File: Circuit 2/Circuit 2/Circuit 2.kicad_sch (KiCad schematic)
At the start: 18 parts, among them SW1 SW_DIP_x08, SW2 SW_DIP_x08, U1 7408, U2 7485, U3 7432

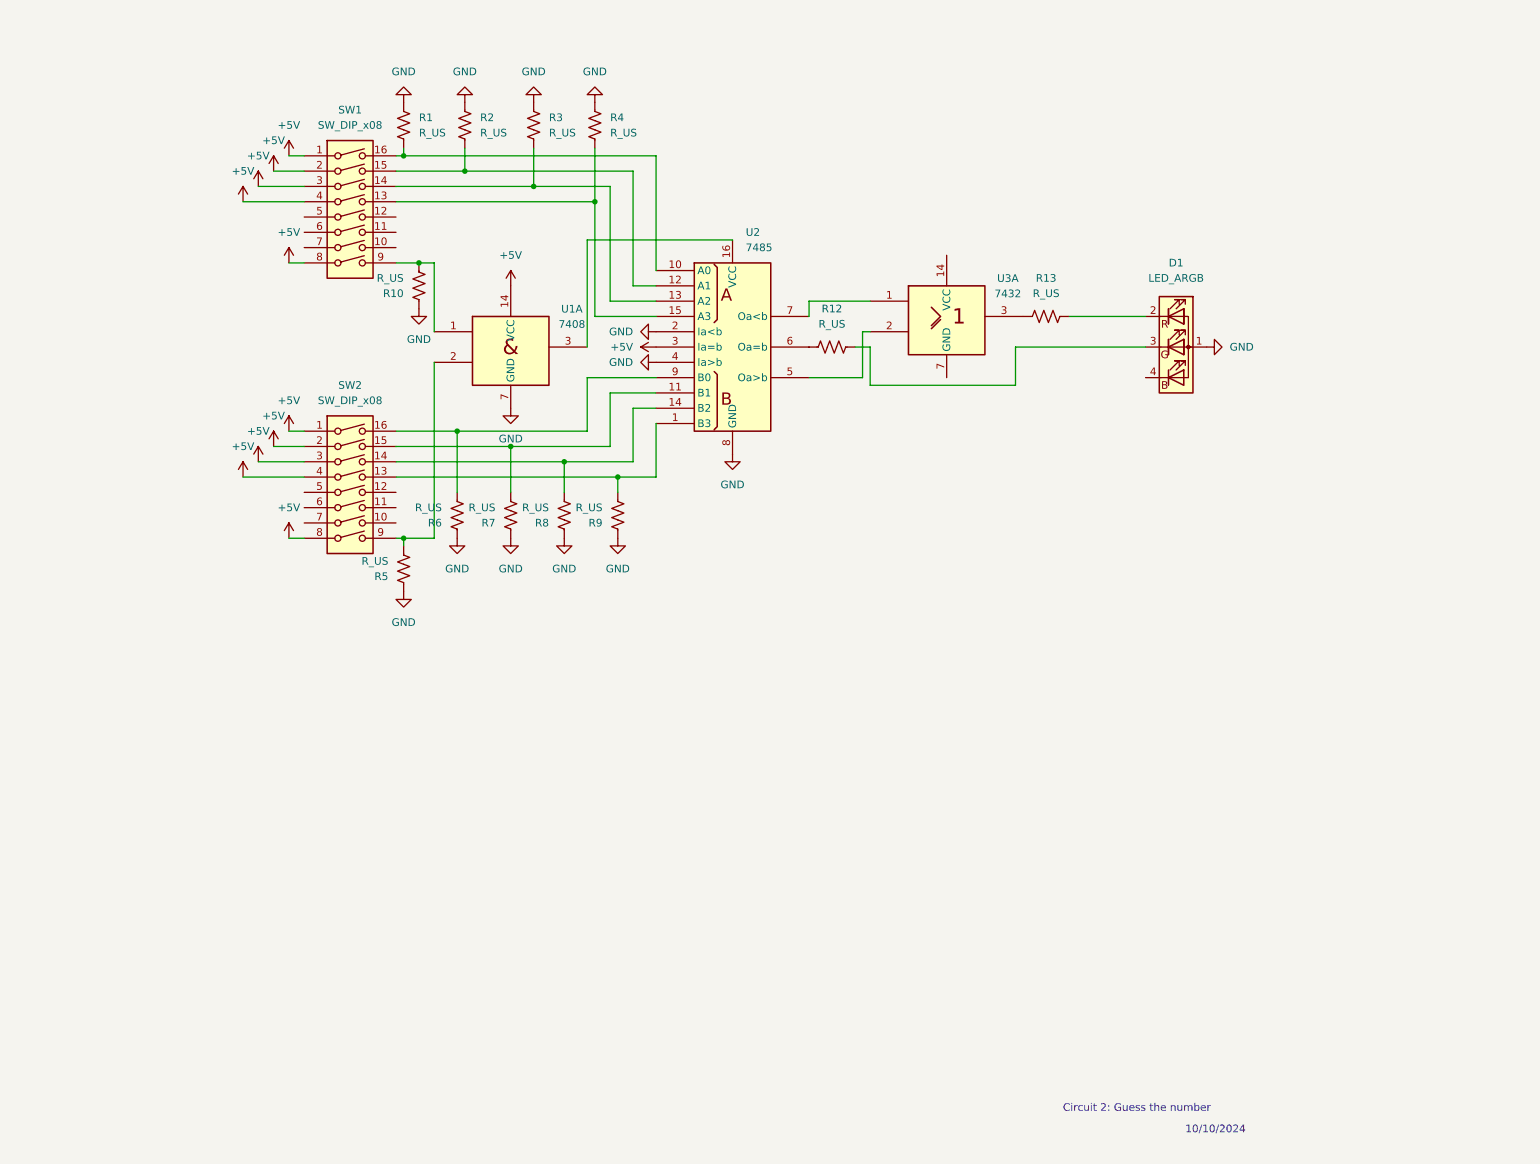
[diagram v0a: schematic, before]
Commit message: Add files via upload
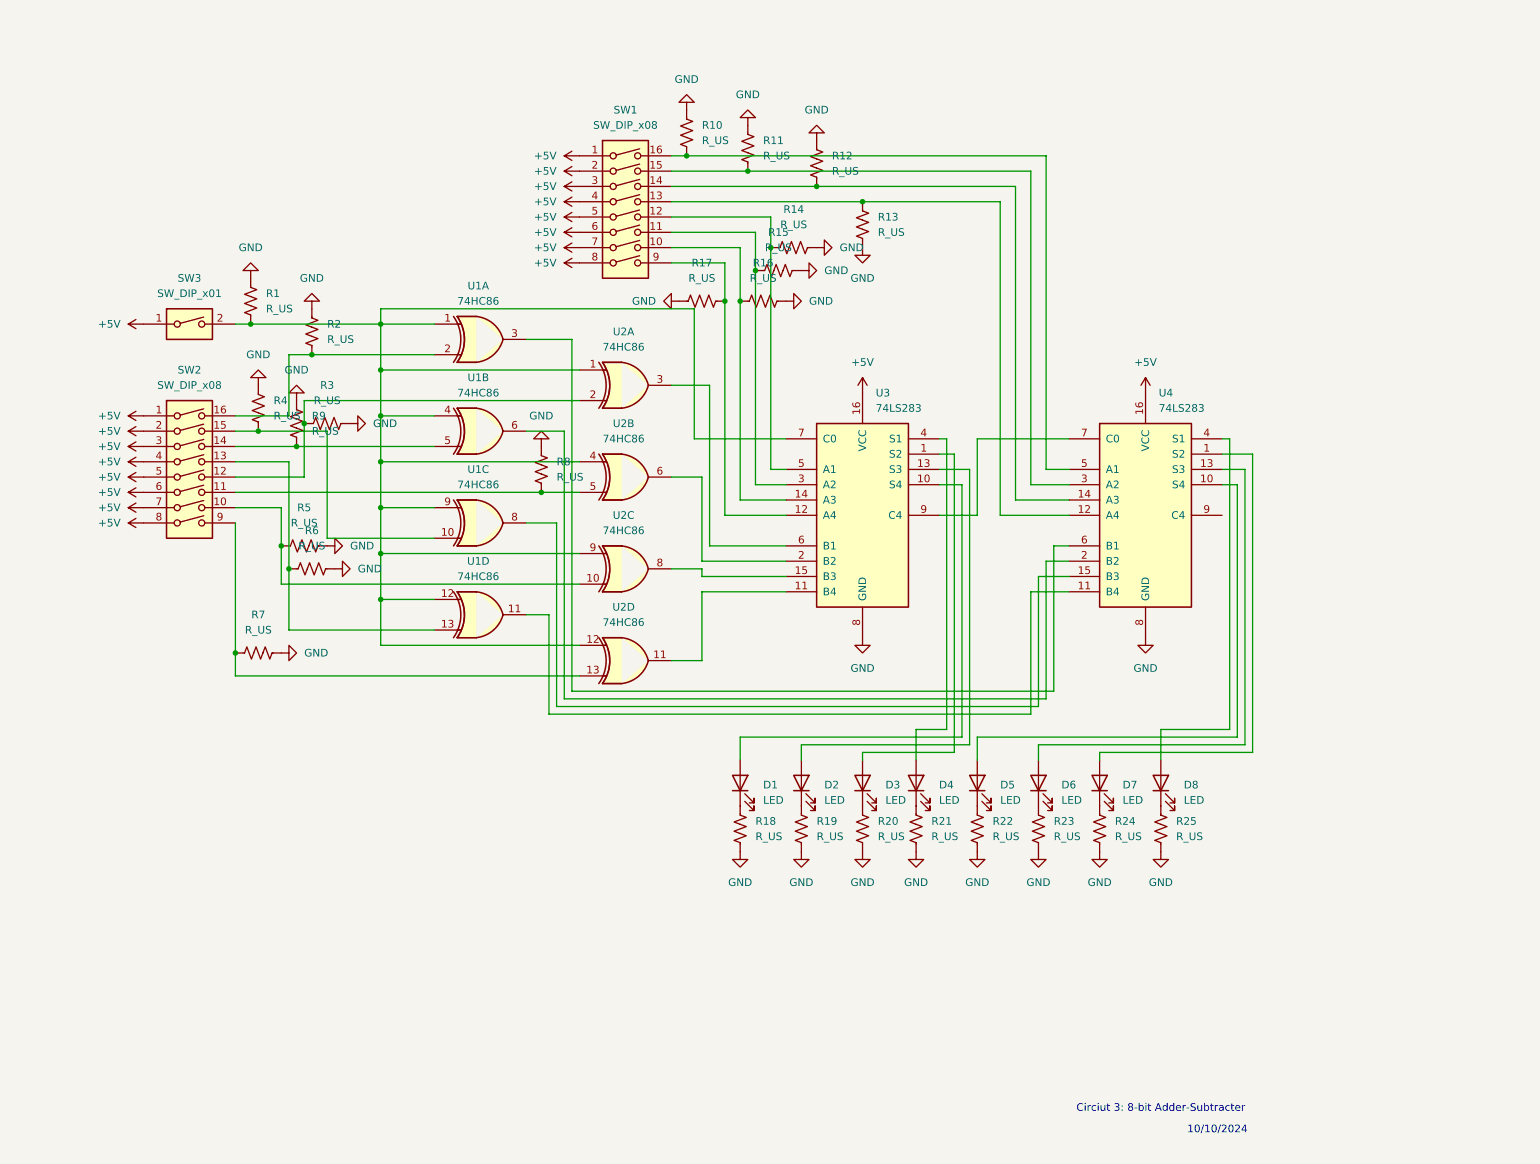
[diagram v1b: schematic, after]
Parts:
- removed D1: LED_ARGB, symbol Device:LED_ARGB
- removed U1: 7408, symbol 74xx_IEEE:7408
- removed U2: 7485, symbol 74xx_IEEE:7485
- removed U3: 7432, symbol 74xx_IEEE:7432
- added D1, D2, D3, D4, D5, D6, D7, D8: LED, symbol Device:LED
- added R11, R14, R15, R16, R17, R18, R19, R20, R21, R22, R23, R24, R25: R_US, symbol Device:R_US
- added SW3: SW_DIP_x01, symbol Switch:SW_DIP_x01
- added U1, U2: 74HC86, symbol 74xx:74HC86
- added U3, U4: 74LS283, symbol 74xx:74LS283
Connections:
- net +5V: now also SW1.5, SW1.6, SW1.7, SW2.5, SW2.6, SW2.7, SW3.1, U3.16 (VCC), U4.16 (VCC)
- net GND: now also R12.1, R13.1, R3.2, R5.2, R6.2, R7.2, R9.2, R11.1, R14.2, R15.2, R16.2, R17.2, R18.2, R19.2, R20.2, R21.2, R22.2, R23.2, R24.2, R25.2, U3.8 (GND), U4.8 (GND); no longer R3.1, R5.1, R6.1, R7.1, R9.1
- net at R13.2: now also SW1.13, U4.12 (A4)
- net at R12.2: now also SW1.14, U4.14 (A3)
- net at R8.2: now also SW2.11, U2.5; no longer SW2.14
- net at SW1.9: now also R17.1, U3.12 (A4); no longer R10.2
- net at SW2.9: now also R7.1, U2.13; no longer R5.2
- net at SW2.13: now also R6.1, U1.13; no longer R9.2
- net at R4.2: now also SW2.15, U1.10; no longer SW1.13
- net at SW2.16: now also R2.2, U1.2; no longer R6.2
- net at SW1.16: now also R10.2, U4.5 (A1); no longer R1.2
- net at SW1.15: now also R11.2, U4.3 (A2); no longer R2.2
- net at SW1.10: now also R16.1, U3.14 (A3)
- net at SW1.11: now also R15.1, U3.3 (A2)
- net at SW1.12: now also R14.1, U3.5 (A1)
- net at SW2.10: now also R5.1, U2.10
- net at SW2.12: now also R3.1, U2.2
- new net: D6.1 (K), R23.1
- new net: D7.2 (A), U4.1 (S2)
- new net: D5.2 (A), U4.10 (S4)
- new net: U1.11, U4.11 (B4)
- new net: D6.2 (A), U4.13 (S3)
- new net: U1.8, U4.15 (B3)
- new net: U1.6, U4.2 (B2)
- new net: D8.2 (A), U4.4 (S1)
- new net: U1.3, U4.6 (B1)
- new net: U3.9 (C4), U4.7 (C0)
- new net: D2.1 (K), R19.1
- new net: R1.2, SW3.2, U1.1, U1.12, U1.4, U1.9, U2.1, U2.12, U2.4, U2.9, U3.7 (C0)
- new net: U2.6, U3.2 (B2)
- new net: D4.1 (K), R21.1
- new net: R9.1, SW2.14, U1.5
- new net: D8.1 (K), R25.1
- new net: U2.3, U3.6 (B1)
- new net: D2.2 (A), U3.13 (S3)
- new net: U2.8, U3.15 (B3)
- new net: D1.1 (K), R18.1
- new net: D1.2 (A), U3.10 (S4)
- new net: D3.1 (K), R20.1
- new net: D3.2 (A), U3.1 (S2)
- new net: D5.1 (K), R22.1
- new net: D7.1 (K), R24.1
- new net: U2.11, U3.11 (B4)
- new net: D4.2 (A), U3.4 (S1)
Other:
- note added: "Circiut 3: 8-bit Adder-Subtracter"
- note removed: "Circuit 2: Guess the number"

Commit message: Add files via upload
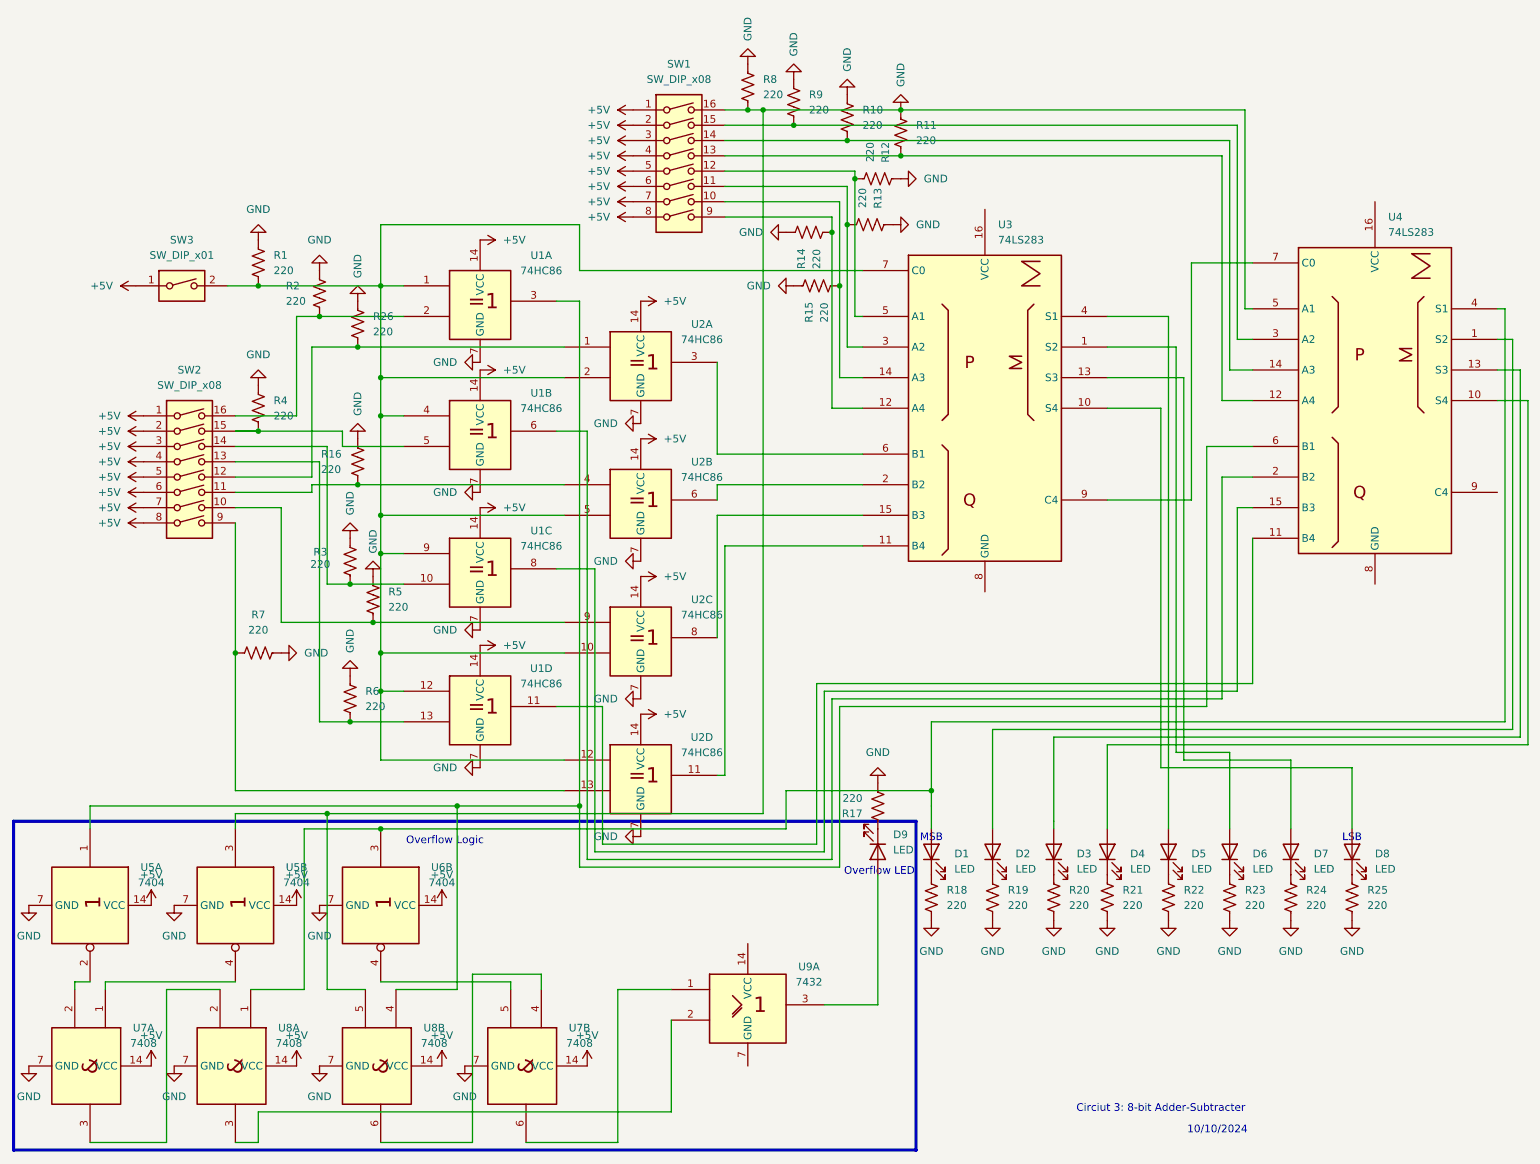
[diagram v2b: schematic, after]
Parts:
- removed U3, U4: 74LS283, symbol 74xx:74LS283
- added D9: LED, symbol Device:LED
- added R26: 220, symbol Device:R_US
- added U3, U4: 74LS283, symbol 74xx_IEEE:74LS283
- added U5, U6: 7404, symbol 74xx_IEEE:7404
- added U7, U8: 7408, symbol 74xx_IEEE:7408
- added U9: 7432, symbol 74xx_IEEE:7432
- R1, R10, R11, R12, R13, R14, R15, R16, R17, R18, R19, R2, R20, R21, R22, R23, R24, R25, R3, R4, R5, R6, R7, R8, R9: value R_US -> 220
- U1, U2: symbol 74xx:74HC86 -> 74xx_IEEE:7486
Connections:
- net +5V: now also U1.14 (VCC), U1.14 (VCC), U1.14 (VCC), U1.14 (VCC), U2.14 (VCC), U2.14 (VCC), U2.14 (VCC), U2.14 (VCC), U5.14 (VCC), U5.14 (VCC), U6.14 (VCC), U7.14 (VCC), U7.14 (VCC), U8.14 (VCC), U8.14 (VCC)
- net GND: now also R10.2, R11.2, R12.2, R13.2, R8.2, SW1.16, U1.7 (GND), U1.7 (GND), U1.7 (GND), U1.7 (GND), U2.7 (GND), U2.7 (GND), U2.7 (GND), U2.7 (GND), R26.2, U4.5 (A1), U5.3, U5.7 (GND), U5.7 (GND), U6.7 (GND), U7.7 (GND), U7.7 (GND), U8.5, U8.7 (GND), U8.7 (GND); no longer R10.1, R11.1, R12.1, R13.1
- net at SW1.9: now also R14.1, U3.12 (A4); no longer R17.1
- net at R16.1: now also SW2.11, U2.4; no longer SW1.10
- net at D7.2 (A): now also U3.13 (S3)
- net at D5.2 (A): now also U3.4 (S1)
- net at U1.11: now also U4.11 (B4)
- net at SW1.13: now also R11.1, U4.12 (A4); no longer R13.2
- net at D6.2 (A): now also U3.1 (S2)
- net at SW1.14: now also R10.1, U4.14 (A3); no longer R12.2
- net at U1.8: now also U4.15 (B3)
- net at U1.6: now also U4.2 (B2)
- net at SW1.15: now also R9.1, U4.3 (A2); no longer R11.2
- net at D8.2 (A): now also U3.10 (S4)
- net at U1.3: now also U4.6 (B1), U5.1, U8.4
- net at R5.1, SW2.10: now also U2.9; no longer U2.10
- net at R1.2, SW3.2, U1.1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: now also U2.10, U2.2, U2.5, U3.7 (C0); no longer U2.1, U2.4, U2.9
- net at U2.6: now also U3.2 (B2)
- net at R15.1: now also SW1.10, U3.14 (A3); no longer SW1.11
- net at SW1.12: now also R12.1, U3.5 (A1); no longer R14.1
- net at R4.2, SW2.15: now also U1.5; no longer U1.10
- net at U2.3: now also U3.6 (B1)
- net at D2.2 (A): now also U4.1 (S2)
- net at U2.8: now also U3.15 (B3)
- net at D1.2 (A): now also U4.4 (S1), U6.3, U8.1
- net at D3.2 (A): now also U4.13 (S3)
- net at U2.11: now also U3.11 (B4)
- net at D4.2 (A): now also U4.10 (S4)
- new net: U5.4, U7.1
- new net: U5.2, U7.2
- new net: U7.3, U8.2
- new net: U7.4, U8.6
- new net: R13.1, SW1.11, U3.3 (A2)
- new net: U6.4, U7.5
- new net: R26.1, SW2.12, U2.1
- new net: R3.1, SW2.14, U1.10
- new net: D9.1 (K), R17.1
- new net: D9.2 (A), U9.3
- new net: U3.9 (C4), U4.7 (C0)
- new net: U7.6, U9.1
- new net: U8.3, U9.2
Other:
- note added: "LSB"
- note added: "MSB"
- note added: "Overflow LED"
- note added: "Overflow Logic"
- moved on the sheet: D1, D2, D3, D4, D5, D6, D7, D8, R1, R18, R19, R2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

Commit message: Add files via upload
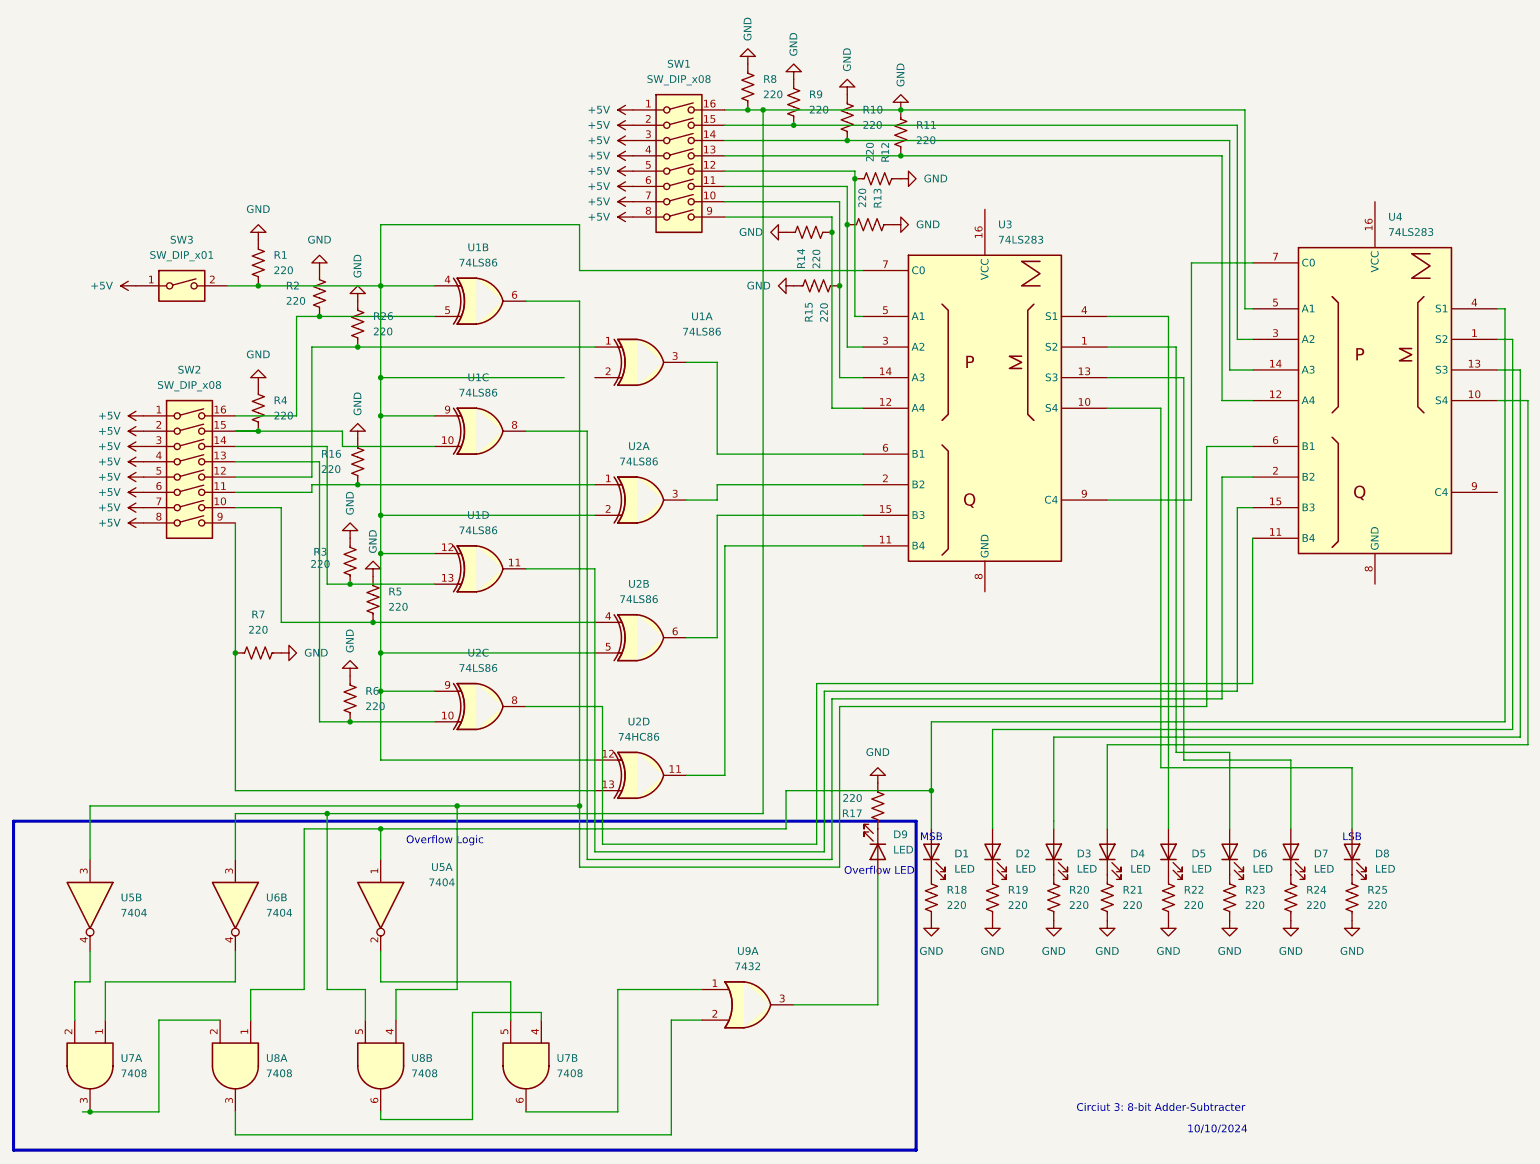
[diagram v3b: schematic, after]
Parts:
- U1, U2: value 74HC86 -> 74LS86; symbol 74xx_IEEE:7486 -> 74xx:74LS86
- U2: symbol 74xx_IEEE:7486 -> 74xx:74LS86
- U5, U6: symbol 74xx_IEEE:7404 -> 74xx:74LS04
- U7, U8: symbol 74xx_IEEE:7408 -> 74xx:74LS08
- U9: symbol 74xx_IEEE:7432 -> 74xx:74LS32
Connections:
- net +5V: no longer U1.14 (VCC), U1.14 (VCC), U1.14 (VCC), U1.14 (VCC), U2.14 (VCC), U2.14 (VCC), U2.14 (VCC), U2.14 (VCC), U5.14 (VCC), U5.14 (VCC), U6.14 (VCC), U7.14 (VCC), U7.14 (VCC), U8.14 (VCC), U8.14 (VCC)
- net GND: now also U6.3; no longer U1.7 (GND), U1.7 (GND), U1.7 (GND), U1.7 (GND), U2.7 (GND), U2.7 (GND), U2.7 (GND), U2.7 (GND), U5.3, U5.7 (GND), U5.7 (GND), U6.7 (GND), U7.7 (GND), U7.7 (GND), U8.7 (GND), U8.7 (GND)
- net at R6.1, SW2.13: now also U2.10; no longer U1.13
- net at U7.1: now also U6.4; no longer U5.4
- net at U7.2: now also U5.4; no longer U5.2
- net at R2.2, SW2.16: now also U1.5; no longer U1.2
- net at R16.1, SW2.11: now also U2.1; no longer U2.4
- net at R1.2, SW3.2, U1.12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: now also U2.9; no longer U1.1, U2.10
- net at U2.6: now also U3.15 (B3); no longer U3.2 (B2)
- net at U4.6 (B1), U8.4: now also U1.6, U5.3; no longer U1.3, U5.1
- net at R5.1, SW2.10: now also U2.4; no longer U2.9
- net at U1.11: now also U4.15 (B3); no longer U4.11 (B4)
- net at D1.2 (A), U4.4 (S1), U8.1: now also U5.1; no longer U6.3
- net at U7.5: now also U5.2; no longer U6.4
- net at R4.2, SW2.15: now also U1.10; no longer U1.5
- net at R26.1, SW2.12: now also U1.1; no longer U2.1
- net at U2.3: now also U3.2 (B2); no longer U3.6 (B1)
- net at R3.1, SW2.14: now also U1.13; no longer U1.10
- net at U1.8: now also U4.2 (B2); no longer U4.15 (B3)
- net at U2.8: now also U4.11 (B4); no longer U3.15 (B3)
- new net: U1.3, U3.6 (B1)
